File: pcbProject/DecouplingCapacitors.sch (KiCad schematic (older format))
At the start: 14 parts

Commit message: deel1routingpcb
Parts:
- C10, C9: footprint (none) -> Capacitor_SMD:CP_Elec_4x3.9
- C11, C12, C13, C16, C17, C18, C4, C5, C7, C8: footprint (none) -> Capacitor_SMD:C_1206_3216Metric
- R11, R12: footprint (none) -> Resistor_SMD:R_1206_3216Metric
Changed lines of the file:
@@
 F 0 "C11" H 2690 2946 50  0000 L CNN
 F 1 "10u" H 2690 2855 50  0000 L CNN
-F 2 "" H 2613 2750 50  0001 C CNN
+F 2 "Capacitor_SMD:C_1206_3216Metric" H 2613 2750 50  0001 C CNN
 F 3 "~" H 2575 2900 50  0001 C CNN
 	1    2575 2900
@@
 F 0 "C12" H 3165 2946 50  0000 L CNN
 F 1 "10u" H 3165 2855 50  0000 L CNN
-F 2 "" H 3088 2750 50  0001 C CNN
+F 2 "Capacitor_SMD:C_1206_3216Metric" H 3088 2750 50  0001 C CNN
 F 3 "~" H 3050 2900 50  0001 C CNN
 	1    3050 2900
@@
 F 0 "C16" H 3965 2946 50  0000 L CNN
 F 1 "100n" H 3965 2855 50  0000 L CNN
-F 2 "" H 3888 2750 50  0001 C CNN
+F 2 "Capacitor_SMD:C_1206_3216Metric" H 3888 2750 50  0001 C CNN
 F 3 "~" H 3850 2900 50  0001 C CNN
 	1    3850 2900
@@
 F 0 "C17" H 4440 2946 50  0000 L CNN
 F 1 "100n" H 4440 2855 50  0000 L CNN
-F 2 "" H 4363 2750 50  0001 C CNN
+F 2 "Capacitor_SMD:C_1206_3216Metric" H 4363 2750 50  0001 C CNN
 F 3 "~" H 4325 2900 50  0001 C CNN
 	1    4325 2900
@@
 F 0 "C18" H 4915 2946 50  0000 L CNN
 F 1 "100n" H 4915 2855 50  0000 L CNN
-F 2 "" H 4838 2750 50  0001 C CNN
+F 2 "Capacitor_SMD:C_1206_3216Metric" H 4838 2750 50  0001 C CNN
 F 3 "~" H 4800 2900 50  0001 C CNN
 	1    4800 2900
@@
 F 0 "C4" H 5365 2946 50  0000 L CNN
 F 1 "100n" H 5365 2855 50  0000 L CNN
-F 2 "" H 5288 2750 50  0001 C CNN
+F 2 "Capacitor_SMD:C_1206_3216Metric" H 5288 2750 50  0001 C CNN
 F 3 "~" H 5250 2900 50  0001 C CNN
 	1    5250 2900
@@
 F 0 "R11" H 2570 4496 50  0000 L CNN
 F 1 "1" H 2570 4405 50  0000 L CNN
-F 2 "" V 2430 4450 50  0001 C CNN
+F 2 "Resistor_SMD:R_1206_3216Metric" V 2430 4450 50  0001 C CNN
 F 3 "~" H 2500 4450 50  0001 C CNN
 	1    2500 4450
@@
 F 0 "R12" H 2970 4496 50  0000 L CNN
 F 1 "1" H 2970 4405 50  0000 L CNN
-F 2 "" V 2830 4450 50  0001 C CNN
+F 2 "Resistor_SMD:R_1206_3216Metric" V 2830 4450 50  0001 C CNN
 F 3 "~" H 2900 4450 50  0001 C CNN
 	1    2900 4450
@@
 F 0 "C5" H 2615 4971 50  0000 L CNN
 F 1 "10u" H 2615 4880 50  0000 L CNN
-F 2 "" H 2538 4775 50  0001 C CNN
+F 2 "Capacitor_SMD:C_1206_3216Metric" H 2538 4775 50  0001 C CNN
 F 3 "~" H 2500 4925 50  0001 C CNN
 	1    2500 4925
@@
 F 0 "C13" H 3015 4971 50  0000 L CNN
 F 1 "10u" H 3015 4880 50  0000 L CNN
-F 2 "" H 2938 4775 50  0001 C CNN
+F 2 "Capacitor_SMD:C_1206_3216Metric" H 2938 4775 50  0001 C CNN
 F 3 "~" H 2900 4925 50  0001 C CNN
 	1    2900 4925
@@
 F 0 "C7" H 4015 4621 50  0000 L CNN
 F 1 "100n" H 4015 4530 50  0000 L CNN
-F 2 "" H 3938 4425 50  0001 C CNN
+F 2 "Capacitor_SMD:C_1206_3216Metric" H 3938 4425 50  0001 C CNN
 F 3 "~" H 3900 4575 50  0001 C CNN
 	1    3900 4575
@@
 F 0 "C8" H 4590 4621 50  0000 L CNN
 F 1 "100n" H 4590 4530 50  0000 L CNN
-F 2 "" H 4513 4425 50  0001 C CNN
+F 2 "Capacitor_SMD:C_1206_3216Metric" H 4513 4425 50  0001 C CNN
 F 3 "~" H 4475 4575 50  0001 C CNN
 	1    4475 4575
@@
 F 0 "C9" H 5243 4621 50  0000 L CNN
 F 1 "0.47u" H 5243 4530 50  0000 L CNN
-F 2 "" H 5163 4425 50  0001 C CNN
+F 2 "Capacitor_SMD:CP_Elec_4x3.9" H 5163 4425 50  0001 C CNN
 F 3 "~" H 5125 4575 50  0001 C CNN
 	1    5125 4575
@@
 F 0 "C10" H 5743 4621 50  0000 L CNN
 F 1 "0.47u" H 5743 4530 50  0000 L CNN
-F 2 "" H 5663 4425 50  0001 C CNN
+F 2 "Capacitor_SMD:CP_Elec_4x3.9" H 5663 4425 50  0001 C CNN
 F 3 "~" H 5625 4575 50  0001 C CNN
 	1    5625 4575

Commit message: PCB versie3
Aanpassingen tips coach --> veel gewijzigd
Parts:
- C11, C12, C13, C16, C17, C18, C4, C5, C7, C8: footprint Capacitor_SMD:C_1206_3216Metric -> Capacitor_SMD:C_1206_3216Metric_Pad1.42x1.75mm_HandSolder
- R11, R12: footprint Resistor_SMD:R_1206_3216Metric -> Resistor_SMD:R_1206_3216Metric_Pad1.42x1.75mm_HandSolder
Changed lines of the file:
@@
 F 0 "C11" H 2690 2946 50  0000 L CNN
 F 1 "10u" H 2690 2855 50  0000 L CNN
-F 2 "Capacitor_SMD:C_1206_3216Metric" H 2613 2750 50  0001 C CNN
+F 2 "Capacitor_SMD:C_1206_3216Metric_Pad1.42x1.75mm_HandSolder" H 2613 2750 50  0001 C CNN
 F 3 "~" H 2575 2900 50  0001 C CNN
 	1    2575 2900
@@
 F 0 "C12" H 3165 2946 50  0000 L CNN
 F 1 "10u" H 3165 2855 50  0000 L CNN
-F 2 "Capacitor_SMD:C_1206_3216Metric" H 3088 2750 50  0001 C CNN
+F 2 "Capacitor_SMD:C_1206_3216Metric_Pad1.42x1.75mm_HandSolder" H 3088 2750 50  0001 C CNN
 F 3 "~" H 3050 2900 50  0001 C CNN
 	1    3050 2900
@@
 F 0 "C16" H 3965 2946 50  0000 L CNN
 F 1 "100n" H 3965 2855 50  0000 L CNN
-F 2 "Capacitor_SMD:C_1206_3216Metric" H 3888 2750 50  0001 C CNN
+F 2 "Capacitor_SMD:C_1206_3216Metric_Pad1.42x1.75mm_HandSolder" H 3888 2750 50  0001 C CNN
 F 3 "~" H 3850 2900 50  0001 C CNN
 	1    3850 2900
@@
 F 0 "C17" H 4440 2946 50  0000 L CNN
 F 1 "100n" H 4440 2855 50  0000 L CNN
-F 2 "Capacitor_SMD:C_1206_3216Metric" H 4363 2750 50  0001 C CNN
+F 2 "Capacitor_SMD:C_1206_3216Metric_Pad1.42x1.75mm_HandSolder" H 4363 2750 50  0001 C CNN
 F 3 "~" H 4325 2900 50  0001 C CNN
 	1    4325 2900
@@
 F 0 "C18" H 4915 2946 50  0000 L CNN
 F 1 "100n" H 4915 2855 50  0000 L CNN
-F 2 "Capacitor_SMD:C_1206_3216Metric" H 4838 2750 50  0001 C CNN
+F 2 "Capacitor_SMD:C_1206_3216Metric_Pad1.42x1.75mm_HandSolder" H 4838 2750 50  0001 C CNN
 F 3 "~" H 4800 2900 50  0001 C CNN
 	1    4800 2900
@@
 F 0 "C4" H 5365 2946 50  0000 L CNN
 F 1 "100n" H 5365 2855 50  0000 L CNN
-F 2 "Capacitor_SMD:C_1206_3216Metric" H 5288 2750 50  0001 C CNN
+F 2 "Capacitor_SMD:C_1206_3216Metric_Pad1.42x1.75mm_HandSolder" H 5288 2750 50  0001 C CNN
 F 3 "~" H 5250 2900 50  0001 C CNN
 	1    5250 2900
@@
 F 0 "R11" H 2570 4496 50  0000 L CNN
 F 1 "1" H 2570 4405 50  0000 L CNN
-F 2 "Resistor_SMD:R_1206_3216Metric" V 2430 4450 50  0001 C CNN
+F 2 "Resistor_SMD:R_1206_3216Metric_Pad1.42x1.75mm_HandSolder" V 2430 4450 50  0001 C CNN
 F 3 "~" H 2500 4450 50  0001 C CNN
 	1    2500 4450
@@
 F 0 "R12" H 2970 4496 50  0000 L CNN
 F 1 "1" H 2970 4405 50  0000 L CNN
-F 2 "Resistor_SMD:R_1206_3216Metric" V 2830 4450 50  0001 C CNN
+F 2 "Resistor_SMD:R_1206_3216Metric_Pad1.42x1.75mm_HandSolder" V 2830 4450 50  0001 C CNN
 F 3 "~" H 2900 4450 50  0001 C CNN
 	1    2900 4450
@@
 F 0 "C5" H 2615 4971 50  0000 L CNN
 F 1 "10u" H 2615 4880 50  0000 L CNN
-F 2 "Capacitor_SMD:C_1206_3216Metric" H 2538 4775 50  0001 C CNN
+F 2 "Capacitor_SMD:C_1206_3216Metric_Pad1.42x1.75mm_HandSolder" H 2538 4775 50  0001 C CNN
 F 3 "~" H 2500 4925 50  0001 C CNN
 	1    2500 4925
@@
 F 0 "C13" H 3015 4971 50  0000 L CNN
 F 1 "10u" H 3015 4880 50  0000 L CNN
-F 2 "Capacitor_SMD:C_1206_3216Metric" H 2938 4775 50  0001 C CNN
+F 2 "Capacitor_SMD:C_1206_3216Metric_Pad1.42x1.75mm_HandSolder" H 2938 4775 50  0001 C CNN
 F 3 "~" H 2900 4925 50  0001 C CNN
 	1    2900 4925
@@
 F 0 "C7" H 4015 4621 50  0000 L CNN
 F 1 "100n" H 4015 4530 50  0000 L CNN
-F 2 "Capacitor_SMD:C_1206_3216Metric" H 3938 4425 50  0001 C CNN
+F 2 "Capacitor_SMD:C_1206_3216Metric_Pad1.42x1.75mm_HandSolder" H 3938 4425 50  0001 C CNN
 F 3 "~" H 3900 4575 50  0001 C CNN
 	1    3900 4575
@@
 F 0 "C8" H 4590 4621 50  0000 L CNN
 F 1 "100n" H 4590 4530 50  0000 L CNN
-F 2 "Capacitor_SMD:C_1206_3216Metric" H 4513 4425 50  0001 C CNN
+F 2 "Capacitor_SMD:C_1206_3216Metric_Pad1.42x1.75mm_HandSolder" H 4513 4425 50  0001 C CNN
 F 3 "~" H 4475 4575 50  0001 C CNN
 	1    4475 4575

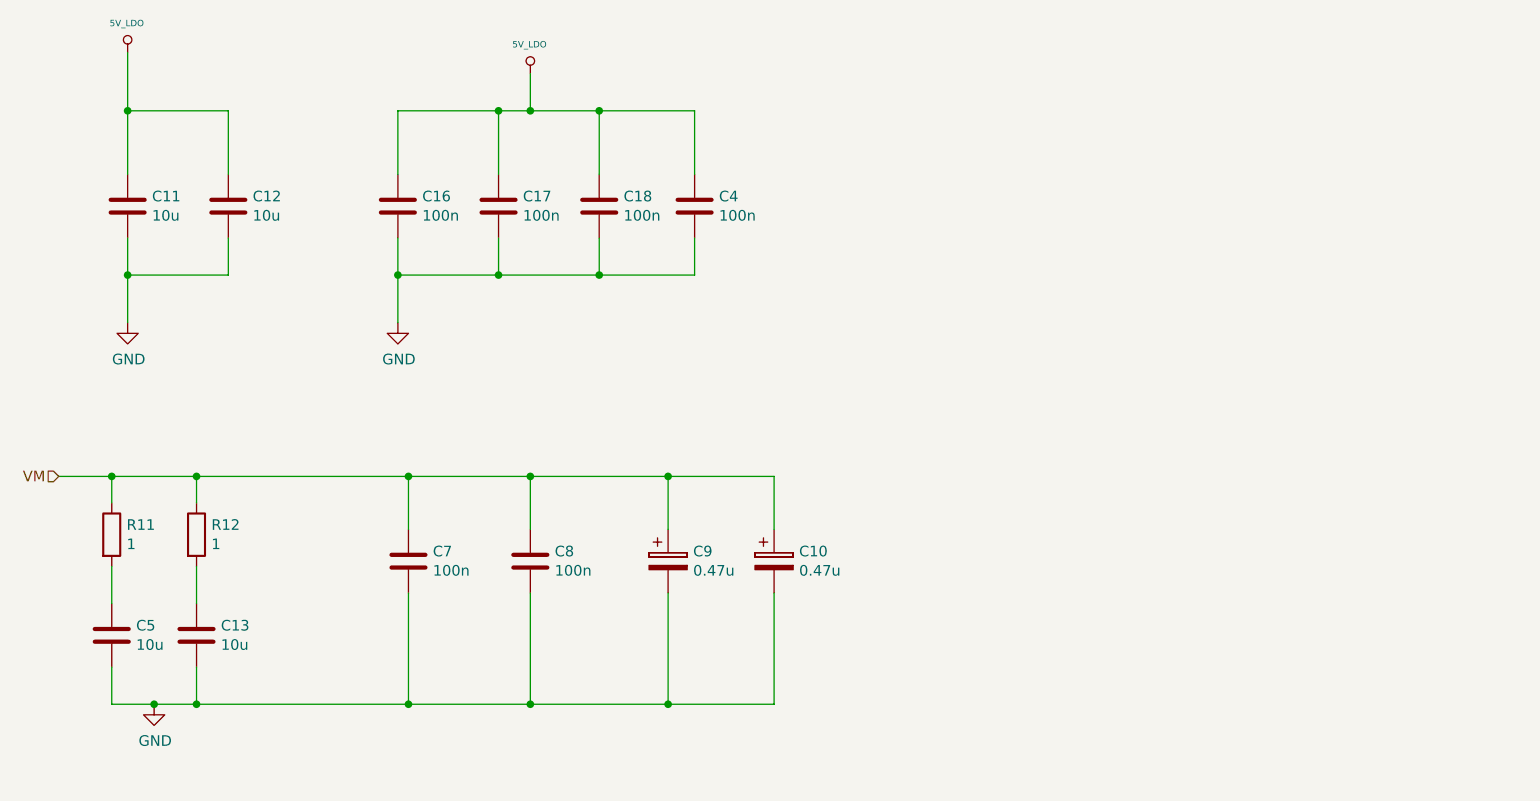
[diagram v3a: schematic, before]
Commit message: verslag
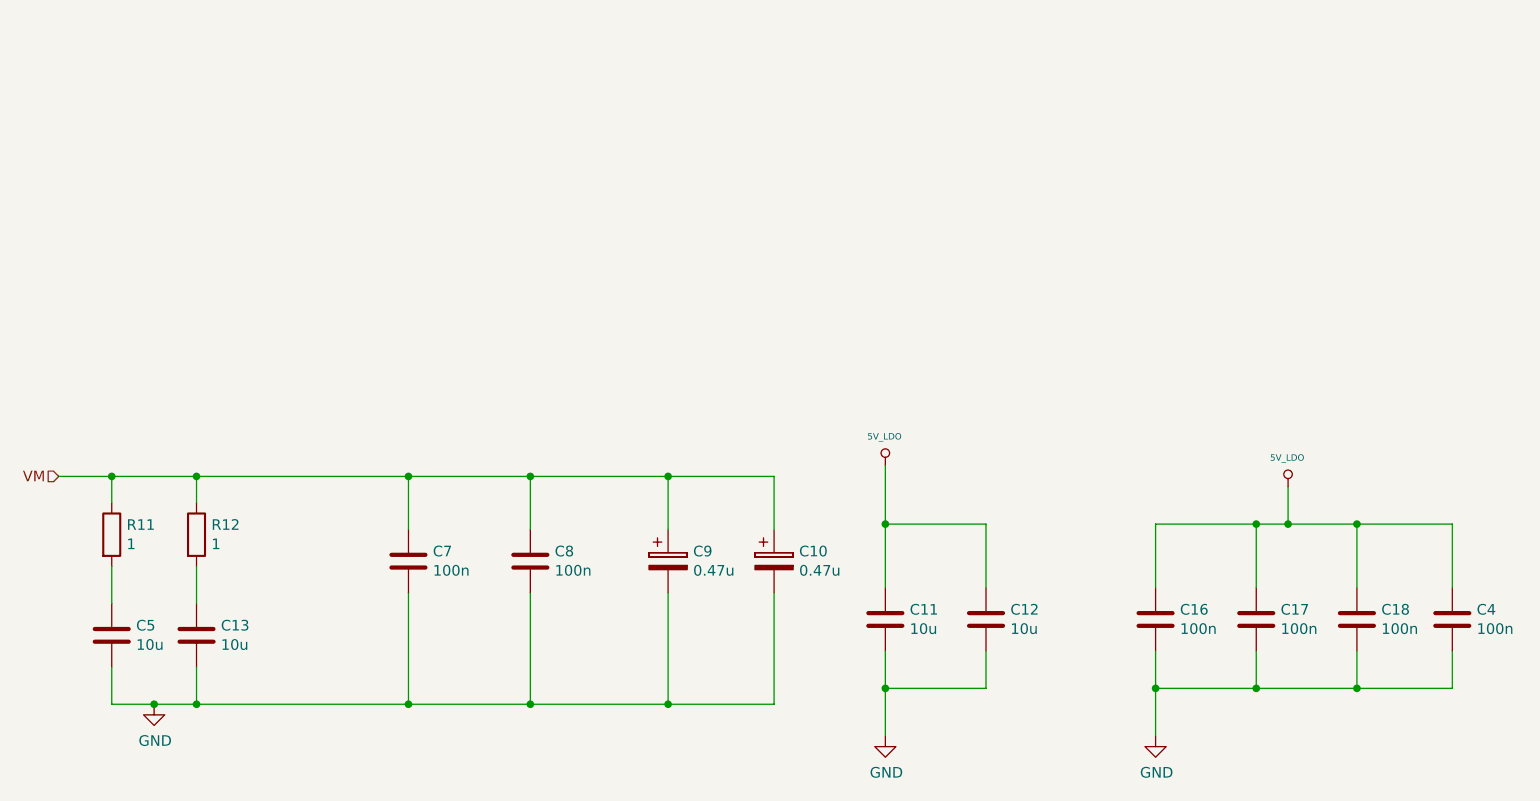
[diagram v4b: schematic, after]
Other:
- moved on the sheet: C11, C12, C16, C17, C18, C4
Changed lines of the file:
@@
 L power:GND #PWR?
 U 1 1 5C78928F
-P 2575 3450
+P 6150 5400
 AR Path="/5C6DA90A/5C78928F" Ref="#PWR?"  Part="1"
 AR Path="/5C6DD8AC/5C78928F" Ref="#PWR0105"  Part="1"
 AR Path="/5C6FDA9D/5C78928F" Ref="#PWR?"  Part="1"
-F 0 "#PWR0105" H 2575 3200 50  0001 C CNN
-F 1 "GND" H 2580 3277 50  0000 C CNN
-F 2 "" H 2575 3450 50  0001 C CNN
-F 3 "" H 2575 3450 50  0001 C CNN
-	1    2575 3450
+F 0 "#PWR0105" H 6150 5150 50  0001 C CNN
+F 1 "GND" H 6155 5227 50  0000 C CNN
+F 2 "" H 6150 5400 50  0001 C CNN
+F 3 "" H 6150 5400 50  0001 C CNN
+	1    6150 5400
 	1    0    0    -1
 $EndComp
@@
 L Arduino_Uno_R3_From_Scratch:5V_LDO #PWR?
 U 1 1 5C789290
-P 2575 2175
+P 6150 4125
 AR Path="/5C6DA90A/5C789290" Ref="#PWR?"  Part="1"
 AR Path="/5C6DD8AC/5C789290" Ref="#PWR0106"  Part="1"
 AR Path="/5C6FDA9D/5C789290" Ref="#PWR?"  Part="1"
-F 0 "#PWR0106" H 2575 2265 20  0001 C CNN
-F 1 "5V_LDO" H 2571 2313 30  0000 C CNN
-F 2 "" H 2575 2175 60  0000 C CNN
-F 3 "" H 2575 2175 60  0000 C CNN
-	1    2575 2175
+F 0 "#PWR0106" H 6150 4215 20  0001 C CNN
+F 1 "5V_LDO" H 6146 4263 30  0000 C CNN
+F 2 "" H 6150 4125 60  0000 C CNN
+F 3 "" H 6150 4125 60  0000 C CNN
+	1    6150 4125
 	1    0    0    -1
 $EndComp
@@
 L Device:C C11
 U 1 1 5C6DE2F5
-P 2575 2900
+P 6150 4850
 AR Path="/5C6DD8AC/5C6DE2F5" Ref="C11"  Part="1"
 AR Path="/5C6FDA9D/5C6DE2F5" Ref="C?"  Part="1"
-F 0 "C11" H 2690 2946 50  0000 L CNN
-F 1 "10u" H 2690 2855 50  0000 L CNN
-F 2 "Capacitor_SMD:C_1206_3216Metric_Pad1.42x1.75mm_HandSolder" H 2613 2750 50  0001 C CNN
-F 3 "~" H 2575 2900 50  0001 C CNN
-	1    2575 2900
+F 0 "C11" H 6265 4896 50  0000 L CNN
+F 1 "10u" H 6265 4805 50  0000 L CNN
+F 2 "Capacitor_SMD:C_1206_3216Metric_Pad1.42x1.75mm_HandSolder" H 6188 4700 50  0001 C CNN
+F 3 "~" H 6150 4850 50  0001 C CNN
+	1    6150 4850
 	1    0    0    -1
 $EndComp
@@
 L Device:C C12
 U 1 1 5C6DE373
-P 3050 2900
+P 6625 4850
 AR Path="/5C6DD8AC/5C6DE373" Ref="C12"  Part="1"
 AR Path="/5C6FDA9D/5C6DE373" Ref="C?"  Part="1"
-F 0 "C12" H 3165 2946 50  0000 L CNN
-F 1 "10u" H 3165 2855 50  0000 L CNN
-F 2 "Capacitor_SMD:C_1206_3216Metric_Pad1.42x1.75mm_HandSolder" H 3088 2750 50  0001 C CNN
-F 3 "~" H 3050 2900 50  0001 C CNN
-	1    3050 2900
+F 0 "C12" H 6740 4896 50  0000 L CNN
+F 1 "10u" H 6740 4805 50  0000 L CNN
+F 2 "Capacitor_SMD:C_1206_3216Metric_Pad1.42x1.75mm_HandSolder" H 6663 4700 50  0001 C CNN
+F 3 "~" H 6625 4850 50  0001 C CNN
+	1    6625 4850
 	1    0    0    -1
 $EndComp
 Wire Wire Line
-	2575 3450 2575 3225
+	6150 5400 6150 5175
 Wire Wire Line
-	2575 2750 2575 2450
+	6150 4700 6150 4400
 Wire Wire Line
-	3050 2750 3050 2450
+	6625 4700 6625 4400
 Wire Wire Line
-	2575 2450 3050 2450
+	6150 4400 6625 4400
 Wire Wire Line
-	3050 3050 3050 3225
+	6625 5000 6625 5175
 Wire Wire Line
-	3050 3225 2575 3225
-Connection ~ 2575 3225
+	6625 5175 6150 5175
+Connection ~ 6150 5175
 Wire Wire Line
-	2575 3225 2575 3050
+	6150 5175 6150 5000
 $Comp
 L power:GND #PWR?
 U 1 1 5C6DE536
-P 3850 3450
+P 7425 5400
 AR Path="/5C6DA90A/5C6DE536" Ref="#PWR?"  Part="1"
 AR Path="/5C6DD8AC/5C6DE536" Ref="#PWR0107"  Part="1"
 AR Path="/5C6FDA9D/5C6DE536" Ref="#PWR?"  Part="1"
-F 0 "#PWR0107" H 3850 3200 50  0001 C CNN
-F 1 "GND" H 3855 3277 50  0000 C CNN
-F 2 "" H 3850 3450 50  0001 C CNN
-F 3 "" H 3850 3450 50  0001 C CNN
-	1    3850 3450
+F 0 "#PWR0107" H 7425 5150 50  0001 C CNN
+F 1 "GND" H 7430 5227 50  0000 C CNN
+F 2 "" H 7425 5400 50  0001 C CNN
+F 3 "" H 7425 5400 50  0001 C CNN
+	1    7425 5400
 	1    0    0    -1
 $EndComp
@@
 L Arduino_Uno_R3_From_Scratch:5V_LDO #PWR?
 U 1 1 5C6DE53C
-P 4475 2275
+P 8050 4225
 AR Path="/5C6DA90A/5C6DE53C" Ref="#PWR?"  Part="1"
 AR Path="/5C6DD8AC/5C6DE53C" Ref="#PWR0108"  Part="1"
 AR Path="/5C6FDA9D/5C6DE53C" Ref="#PWR?"  Part="1"
-F 0 "#PWR0108" H 4475 2365 20  0001 C CNN
-F 1 "5V_LDO" H 4471 2413 30  0000 C CNN
-F 2 "" H 4475 2275 60  0000 C CNN
-F 3 "" H 4475 2275 60  0000 C CNN
-	1    4475 2275
+F 0 "#PWR0108" H 8050 4315 20  0001 C CNN
+F 1 "5V_LDO" H 8046 4363 30  0000 C CNN
+F 2 "" H 8050 4225 60  0000 C CNN
+F 3 "" H 8050 4225 60  0000 C CNN
+	1    8050 4225
 	1    0    0    -1
 $EndComp
 Wire Wire Line
-	4475 2275 4475 2450
+	8050 4225 8050 4400
 $Comp
 L Device:C C16
 U 1 1 5C6DE543
-P 3850 2900
+P 7425 4850
 AR Path="/5C6DD8AC/5C6DE543" Ref="C16"  Part="1"
 AR Path="/5C6FDA9D/5C6DE543" Ref="C?"  Part="1"
-F 0 "C16" H 3965 2946 50  0000 L CNN
-F 1 "100n" H 3965 2855 50  0000 L CNN
-F 2 "Capacitor_SMD:C_1206_3216Metric_Pad1.42x1.75mm_HandSolder" H 3888 2750 50  0001 C CNN
-F 3 "~" H 3850 2900 50  0001 C CNN
-	1    3850 2900
+F 0 "C16" H 7540 4896 50  0000 L CNN
+F 1 "100n" H 7540 4805 50  0000 L CNN
+F 2 "Capacitor_SMD:C_1206_3216Metric_Pad1.42x1.75mm_HandSolder" H 7463 4700 50  0001 C CNN
+F 3 "~" H 7425 4850 50  0001 C CNN
+	1    7425 4850
 	1    0    0    -1
 $EndComp
@@
 L Device:C C17
 U 1 1 5C6DE54A
-P 4325 2900
+P 7900 4850
 AR Path="/5C6DD8AC/5C6DE54A" Ref="C17"  Part="1"
 AR Path="/5C6FDA9D/5C6DE54A" Ref="C?"  Part="1"
-F 0 "C17" H 4440 2946 50  0000 L CNN
-F 1 "100n" H 4440 2855 50  0000 L CNN
-F 2 "Capacitor_SMD:C_1206_3216Metric_Pad1.42x1.75mm_HandSolder" H 4363 2750 50  0001 C CNN
-F 3 "~" H 4325 2900 50  0001 C CNN
-	1    4325 2900
+F 0 "C17" H 8015 4896 50  0000 L CNN
+F 1 "100n" H 8015 4805 50  0000 L CNN
+F 2 "Capacitor_SMD:C_1206_3216Metric_Pad1.42x1.75mm_HandSolder" H 7938 4700 50  0001 C CNN
+F 3 "~" H 7900 4850 50  0001 C CNN
+	1    7900 4850
 	1    0    0    -1
 $EndComp
 Wire Wire Line
-	3850 3450 3850 3225
+	7425 5400 7425 5175
 Wire Wire Line
-	3850 2750 3850 2450
+	7425 4700 7425 4400
 Wire Wire Line
-	4325 2750 4325 2450
+	7900 4700 7900 4400
 Wire Wire Line
-	3850 2450 4325 2450
-Connection ~ 4325 2450
+	7425 4400 7900 4400
+Connection ~ 7900 4400
 Wire Wire Line
-	4325 2450 4475 2450
+	7900 4400 8050 4400
 Wire Wire Line
-	4325 3050 4325 3225
+	7900 5000 7900 5175
 Wire Wire Line
-	4325 3225 3850 3225
-Connection ~ 3850 3225
+	7900 5175 7425 5175
+Connection ~ 7425 5175
 Wire Wire Line
-	3850 3225 3850 3050
+	7425 5175 7425 5000
 $Comp
 L Device:C C18
 U 1 1 5C6DE722
-P 4800 2900
+P 8375 4850
 AR Path="/5C6DD8AC/5C6DE722" Ref="C18"  Part="1"
 AR Path="/5C6FDA9D/5C6DE722" Ref="C?"  Part="1"
-F 0 "C18" H 4915 2946 50  0000 L CNN
-F 1 "100n" H 4915 2855 50  0000 L CNN
-F 2 "Capacitor_SMD:C_1206_3216Metric_Pad1.42x1.75mm_HandSolder" H 4838 2750 50  0001 C CNN
-F 3 "~" H 4800 2900 50  0001 C CNN
-	1    4800 2900
+F 0 "C18" H 8490 4896 50  0000 L CNN
+F 1 "100n" H 8490 4805 50  0000 L CNN
+F 2 "Capacitor_SMD:C_1206_3216Metric_Pad1.42x1.75mm_HandSolder" H 8413 4700 50  0001 C CNN
+F 3 "~" H 8375 4850 50  0001 C CNN
+	1    8375 4850
 	1    0    0    -1
 $EndComp
 Wire Wire Line
-	4800 2750 4800 2450
+	8375 4700 8375 4400
 Wire Wire Line
-	4800 3050 4800 3225
+	8375 5000 8375 5175
 $Comp
 L Device:C C4
 U 1 1 5C6DE8B0
-P 5250 2900
+P 8825 4850
 AR Path="/5C6DD8AC/5C6DE8B0" Ref="C4"  Part="1"
 AR Path="/5C6FDA9D/5C6DE8B0" Ref="C?"  Part="1"
-F 0 "C4" H 5365 2946 50  0000 L CNN
-F 1 "100n" H 5365 2855 50  0000 L CNN
-F 2 "Capacitor_SMD:C_1206_3216Metric_Pad1.42x1.75mm_HandSolder" H 5288 2750 50  0001 C CNN
-F 3 "~" H 5250 2900 50  0001 C CNN
-	1    5250 2900
+F 0 "C4" H 8940 4896 50  0000 L CNN
+F 1 "100n" H 8940 4805 50  0000 L CNN
+F 2 "Capacitor_SMD:C_1206_3216Metric_Pad1.42x1.75mm_HandSolder" H 8863 4700 50  0001 C CNN
+F 3 "~" H 8825 4850 50  0001 C CNN
+	1    8825 4850
 	1    0    0    -1
 $EndComp
 Wire Wire Line
-	5250 2750 5250 2450
+	8825 4700 8825 4400
 Wire Wire Line
-	5250 3050 5250 3225
+	8825 5000 8825 5175
 Wire Wire Line
-	4475 2450 4800 2450
-Connection ~ 4475 2450
+	8050 4400 8375 4400
+Connection ~ 8050 4400
 Wire Wire Line
-	4800 2450 5250 2450
-Connection ~ 4800 2450
+	8375 4400 8825 4400
+Connection ~ 8375 4400
 Wire Wire Line
-	4800 3225 4325 3225
-Connection ~ 4325 3225
+	8375 5175 7900 5175
+Connection ~ 7900 5175
 Wire Wire Line
-	5250 3225 4800 3225
-Connection ~ 4800 3225
+	8825 5175 8375 5175
+Connection ~ 8375 5175
 Wire Wire Line
-	2575 2175 2575 2450
-Connection ~ 2575 2450
+	6150 4125 6150 4400
+Connection ~ 6150 4400
 Text HLabel 2250 4175 0    50   Input ~ 0
 VM
